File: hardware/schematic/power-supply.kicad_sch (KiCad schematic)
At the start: 27 parts, among them J1 VIN_IN, Q1 IRFR4615, U1 LM5164DDA, U2 AMS1117-5.0, U3 AMS1117-3.3

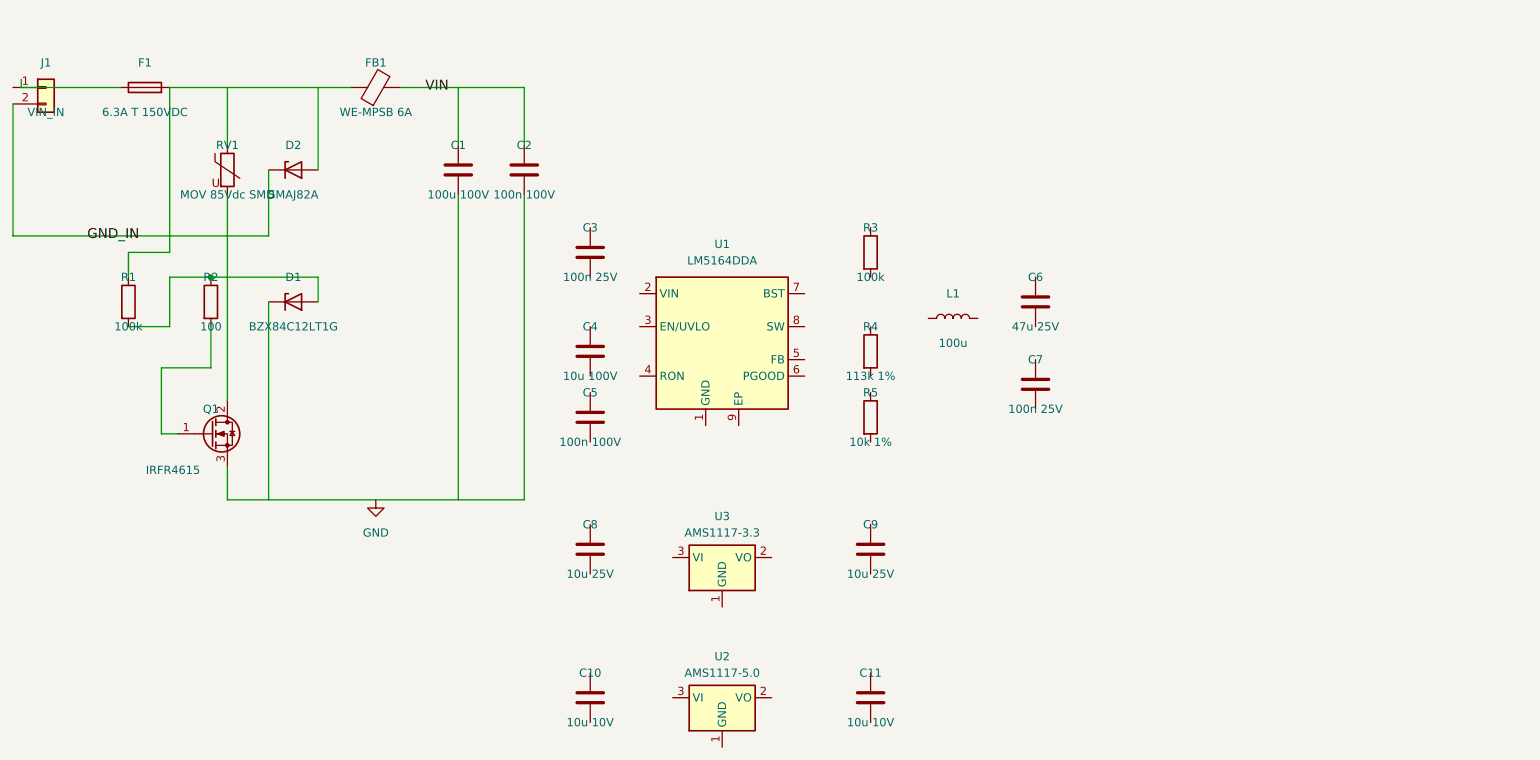
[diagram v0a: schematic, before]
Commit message: updates
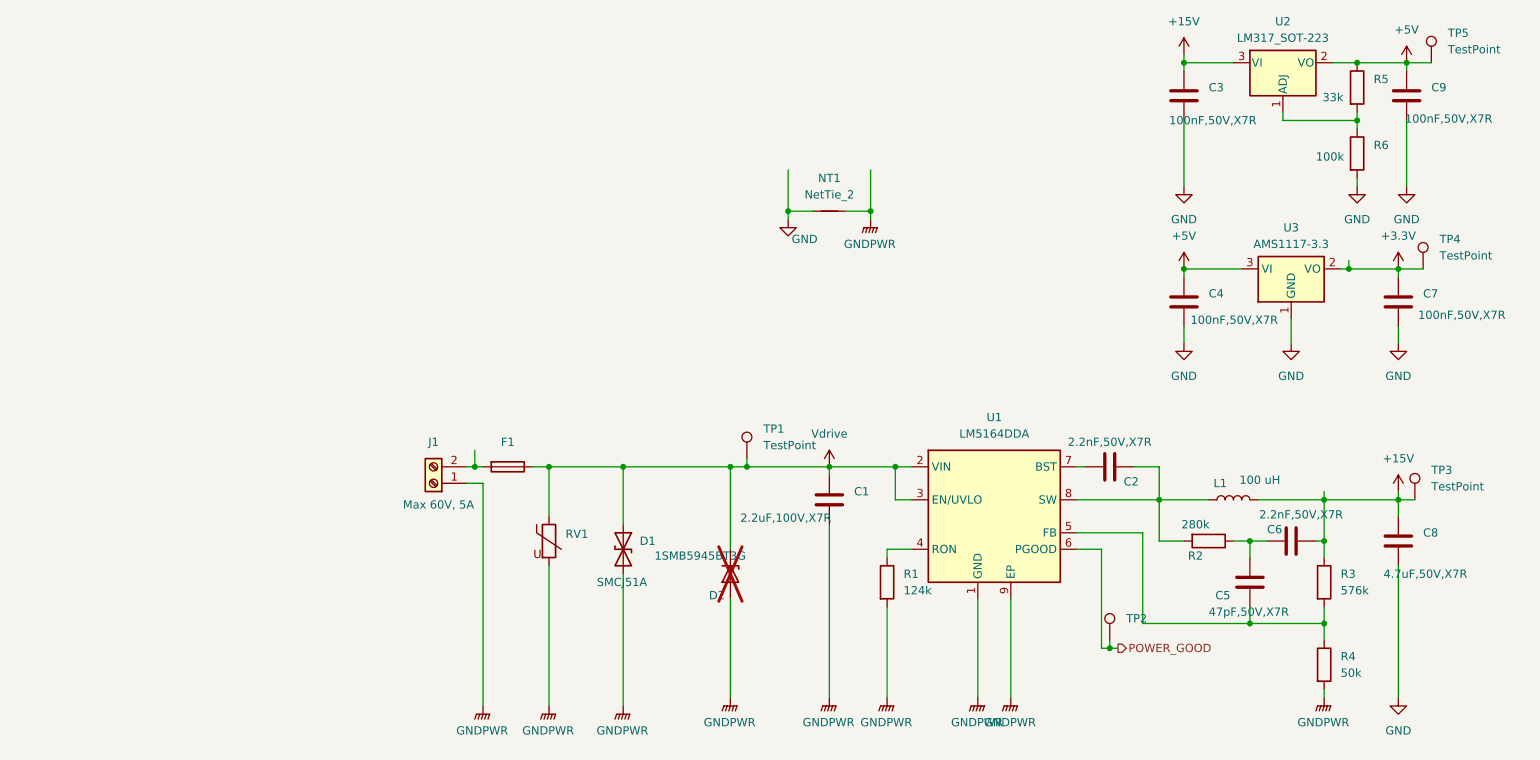
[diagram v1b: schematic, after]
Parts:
- removed C10, C11: 10u 10V, Capacitor_SMD:C_0805_2012Metric, symbol Device:C
- removed D1: BZX84C12LT1G, Diode_SMD:D_SOD-123, symbol Device:D_Zener
- removed FB1: WE-MPSB 6A, Inductor_SMD:L_1812_4532Metric_HandSolder, symbol Device:FerriteBead
- removed J1: VIN_IN, TerminalBlock_Phoenix:TerminalBlock_Phoenix_PT-1,5-2-3.5_1x02_P3.50mm_Horizontal, symbol Connector_Generic:Conn_01x02
- removed Q1: IRFR4615, Package_TO_SOT_SMD:TO-252-3_TabPin2, symbol Transistor_FET:Q_NMOS_GDS
- removed U2: AMS1117-5.0, Package_TO_SOT_SMD:SOT-223-3_TabPin2, symbol Regulator_Linear:AMS1117-5.0
- added D1: SMCJ51A, Diode_SMD:D_SMC, symbol Device:D_TVS
- added J1: Screw_Terminal_01x02, TerminalBlock_CUI:TerminalBlock_CUI_TB007-508-02_1x02_P5.08mm_Horizontal, symbol Connector:Screw_Terminal_01x02
- added NT1: NetTie_2, NetTie:NetTie-2_SMD_Pad2.0mm, symbol Device:NetTie_2
- added R6: 100k, Resistor_SMD:R_0805_2012Metric_Pad1.20x1.40mm_HandSolder, symbol Device:R
- added TP1, TP2, TP3, TP4, TP5: TestPoint, TestPoint:TestPoint_Pad_1.0x1.0mm, symbol Connector:TestPoint
- added U2: LM317_SOT-223, Package_TO_SOT_SMD:SOT-223-3_TabPin2, symbol Regulator_Linear:LM317_SOT-223
- C1: value 100u 100V -> 2.2uF,100V,X7R; footprint Capacitor_SMD:C_1210_3225Metric -> Capacitor_SMD:C_0805_2012Metric_Pad1.18x1.45mm_HandSolder
- C2: value 100n 100V -> 2.2nF,50V,X7R; footprint Capacitor_SMD:C_0805_2012Metric -> Capacitor_SMD:C_0805_2012Metric_Pad1.18x1.45mm_HandSolder
- C3, C7: value 100n 25V -> 100nF,50V,X7R; footprint Capacitor_SMD:C_0805_2012Metric -> Capacitor_SMD:C_0805_2012Metric_Pad1.18x1.45mm_HandSolder
- C4: value 10u 100V -> 100nF,50V,X7R; footprint Capacitor_SMD:C_1210_3225Metric -> Capacitor_SMD:C_0805_2012Metric_Pad1.18x1.45mm_HandSolder
- C5: value 100n 100V -> 47pF,50V,X7R; footprint Capacitor_SMD:C_0805_2012Metric -> Capacitor_SMD:C_0805_2012Metric_Pad1.18x1.45mm_HandSolder
- C6: value 47u 25V -> 2.2nF,50V,X7R; footprint Capacitor_SMD:C_1210_3225Metric -> Capacitor_SMD:C_0805_2012Metric_Pad1.18x1.45mm_HandSolder
- C8: value 10u 25V -> 4.7uF,50V,X7R; footprint Capacitor_SMD:C_1206_3216Metric -> Capacitor_SMD:C_0805_2012Metric_Pad1.18x1.45mm_HandSolder
- C9: value 10u 25V -> 100nF,50V,X7R; footprint Capacitor_SMD:C_1206_3216Metric -> Capacitor_SMD:C_0805_2012Metric_Pad1.18x1.45mm_HandSolder
- D2: value SMAJ82A -> 1SMB5945BT3G; footprint Diode_SMD:D_SMA -> Diode_SMD:D_SMB; now not fitted
- F1: value 6.3A T 150VDC -> Fuse; footprint Fuse:Fuse_Schurter_UMT250 -> Fuse:Fuse_1812_4532Metric
- L1: value 100u -> 100 uH; footprint Inductor_SMD:L_Bourns_SRR1260 -> Inductor_SMD:L_7.3x7.3_H4.5
- R1: value 100k -> 124k; footprint Resistor_SMD:R_0805_2012Metric -> Resistor_SMD:R_0805_2012Metric_Pad1.20x1.40mm_HandSolder
- R2: value 100 -> 280k; footprint Resistor_SMD:R_0805_2012Metric -> Resistor_SMD:R_0805_2012Metric_Pad1.20x1.40mm_HandSolder
- R3: value 100k -> 576k; footprint Resistor_SMD:R_0805_2012Metric -> Resistor_SMD:R_0805_2012Metric_Pad1.20x1.40mm_HandSolder
- R4: value 113k 1% -> 50k; footprint Resistor_SMD:R_0805_2012Metric -> Resistor_SMD:R_0805_2012Metric_Pad1.20x1.40mm_HandSolder
- R5: value 10k 1% -> 33k; footprint Resistor_SMD:R_0805_2012Metric -> Resistor_SMD:R_0805_2012Metric_Pad1.20x1.40mm_HandSolder
- RV1: value MOV 85Vdc SMD -> Varistor; footprint Varistor:Varistor_Panasonic_VF -> Fuse:Fuse_1812_4532Metric
- U1: footprint Package_SO:HSOP-8-1EP_3.9x4.9mm_P1.27mm_EP2.41x3.1mm_ThermalVias -> Package_SO:HSOP-8-1EP_3.9x4.9mm_P1.27mm_EP2.41x3.1mm
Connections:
- net GND_IN is gone; now on net Vdrive: D2.1 (K)
- net VIN is gone; now on an unnamed net: C2.1
- net GND: now also C3.2, C4.2, C7.2, C8.2, C9.2, U3.1 (GND), NT1.1, R6.2
- net at R4.1: now also C5.2, R3.2, U1.5 (FB)
- net GNDPWR: now reaches R4.2
- net GNDPWR: now also C1.2, D2.2 (A), R1.2, RV1.2, U1.1 (GND), U1.9 (EP), D1.2 (A2), J1.1 (Pin_1), NT1.2
- net +3.3V: now reaches C7.1
- net +3.3V: now also U3.2 (VO), TP4.1
- net at R1.1: now also U1.4 (RON); no longer F1.2
- net at R2.1: now also C5.1, C6.2; no longer R1.2
- net Vdrive: now reaches F1.1
- net Vdrive: now also C1.1, RV1.1, U1.2 (VIN), U1.3 (EN/UVLO), D1.1 (A1), TP1.1
- net +5V: now reaches C4.1
- net +5V: now also C9.1, R5.1, U3.3 (VI), TP5.1, U2.2 (VO)
- net at R2.2: now also L1.1, U1.8 (SW)
- net at C2.2: now also U1.7 (BST)
- net +15V: now reaches C3.1
- net +15V: now also C6.1, C8.1, L1.2, R3.1, TP3.1, U2.3 (VI)
- net POWER_GOOD: now reaches U1.6 (PGOOD)
- net POWER_GOOD: now also TP2.1
- net at R5.2: now also R6.1, U2.1 (ADJ)
- new net: F1.2, J1.2 (Pin_2)
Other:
- moved on the sheet: U1, U3
